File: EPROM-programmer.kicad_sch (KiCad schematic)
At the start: 63 parts, among them J1 ZIF-socket, J2 ISP, J3 DAC_VCC, J4 DAC_B, J5 GND, J6 Barrel_Jack_Switch, J7 VCC_SEL, J8 AMP_VCC, J9 GND, P1 USB-C, Q1 TIP41C, Q2 BC327, Q3 BC337, SW1 SW_Push, U1 ATmega1284-P, U2 MCP2221AxP, U3 MCP4812, U4 LM358, Y1 20M

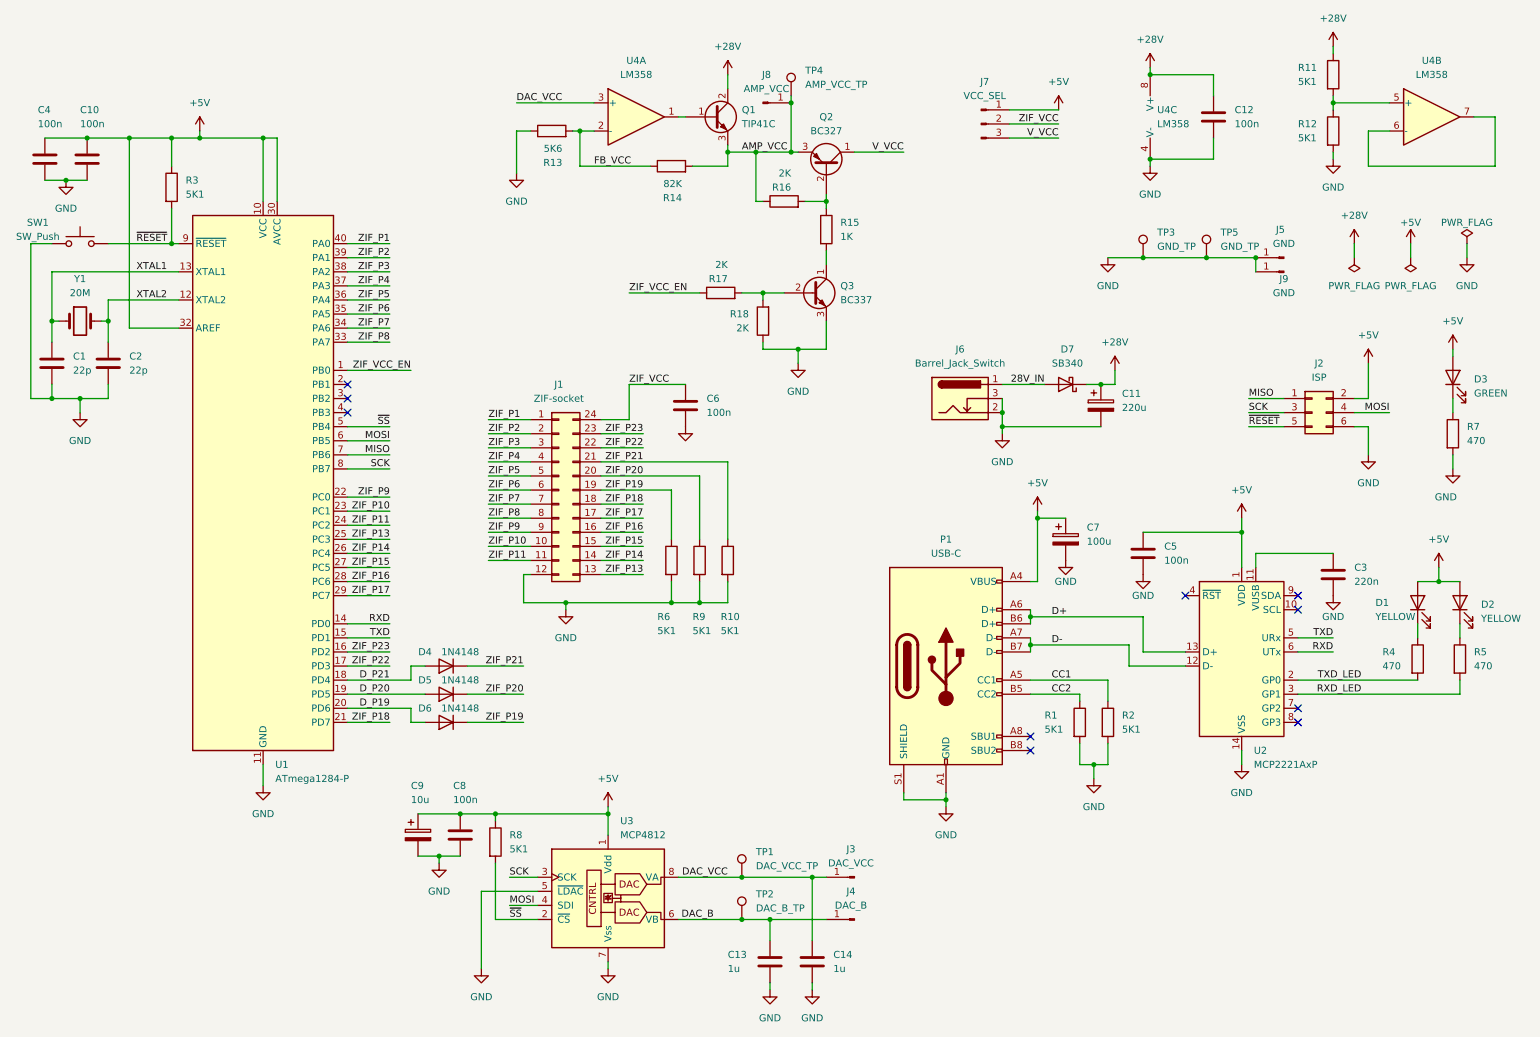
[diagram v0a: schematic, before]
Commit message: WIP use LM317
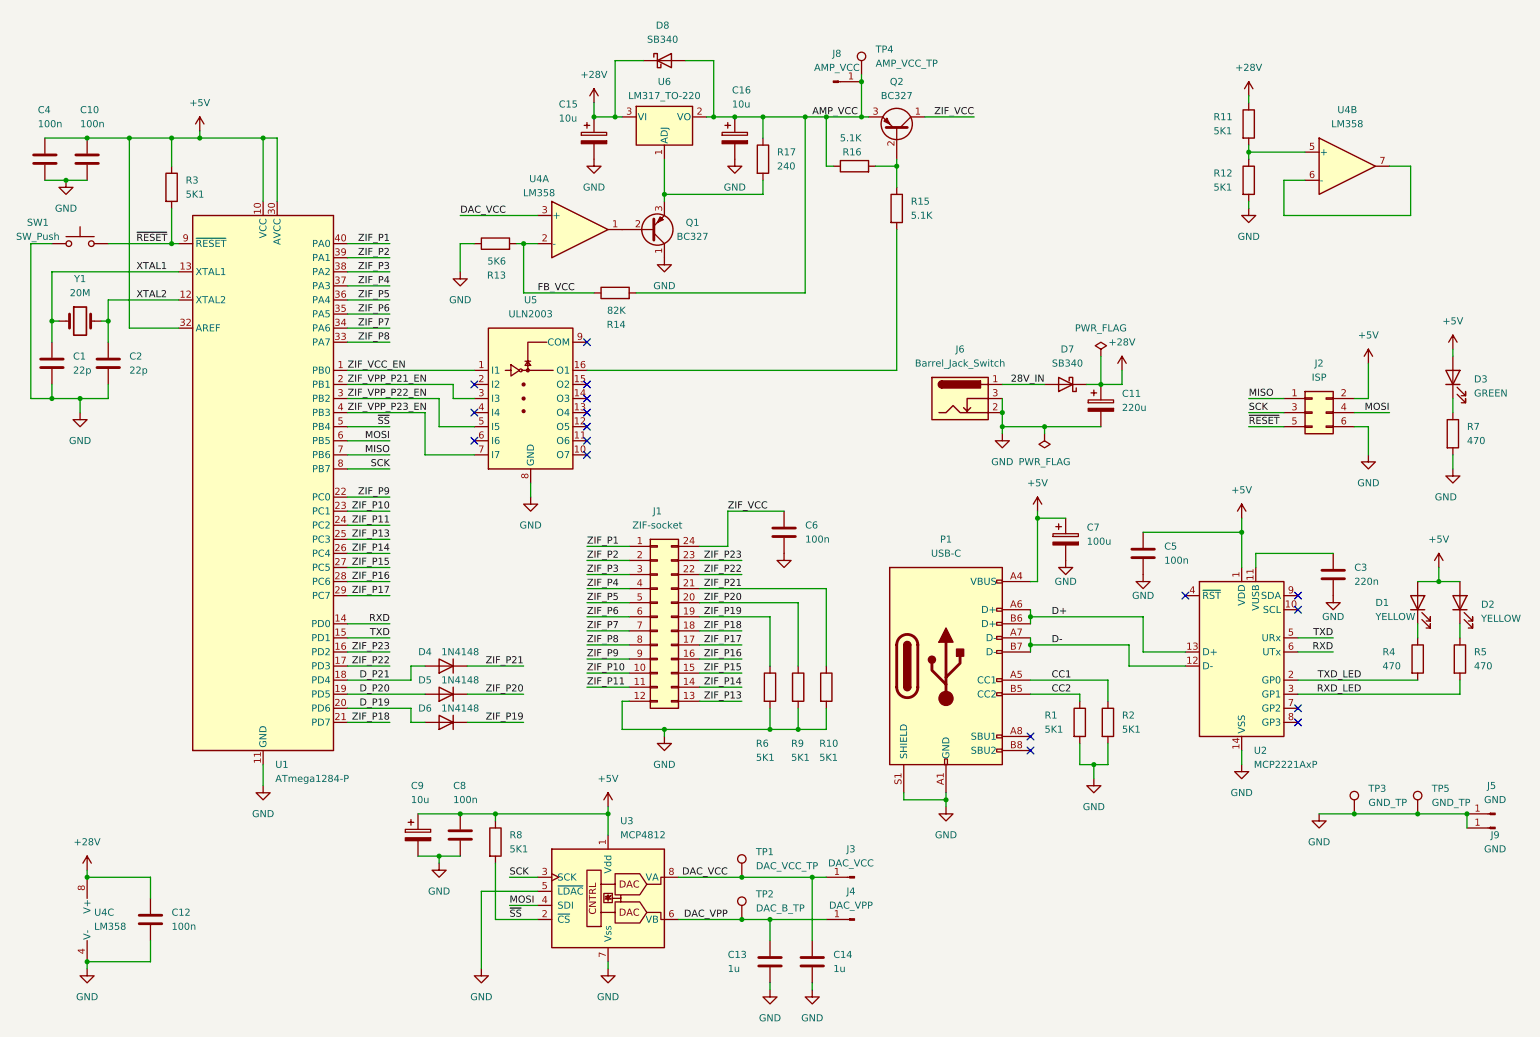
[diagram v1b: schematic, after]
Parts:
- removed J7: VCC_SEL, Connector_PinHeader_2.54mm:PinHeader_1x03_P2.54mm_Vertical, symbol Connector:Conn_01x03_Pin
- removed Q1: TIP41C, Package_TO_SOT_THT:TO-220-3_Vertical, symbol Transistor_BJT:TIP41C
- removed Q3: BC337, Package_TO_SOT_THT:TO-92_Inline_Wide, symbol Transistor_BJT:BC337
- removed R18: 2K, Resistor_THT:R_Axial_DIN0207_L6.3mm_D2.5mm_P10.16mm_Horizontal, symbol Device:R
- added C15, C16: 10u, Local:C_Rect_L4.6mm_W3.0mm_P2.50mm_MKS02_FKP02, symbol Device:C_Polarized
- added D8: SB340, Diode_THT:D_DO-201AD_P15.24mm_Horizontal, symbol Diode:B340
- added Q1: BC327, Package_TO_SOT_THT:TO-92_Inline_Wide, symbol Transistor_BJT:BC327
- added U5: ULN2003, Package_DIP:DIP-16_W7.62mm_Socket, symbol Transistor_Array:ULN2003
- added U6: LM317_TO-220, Package_TO_SOT_THT:TO-220-3_Vertical, symbol Regulator_Linear:LM317_TO-220
- J4: value DAC_B -> DAC_VPP
- R15: value 1K -> 5.1K
- R16: value 2K -> 5.1K
- R17: value 2K -> 240
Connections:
- net V_VCC is gone; now on net ZIF_VCC: Q2.1 (C)
- net +28V: now also C15.1, D8.1 (K), U6.3 (VI)
- net AMP_VCC: now also R17.1, C16.1, D8.2 (A), U6.2 (VO)
- net GND: now also C15.2, C16.2, Q1.1 (C), U5.8 (GND)
- net ZIF_VCC_EN: now also U5.1 (I1); no longer R17.1
- net ZIF_VPP_P21_EN: now reaches U1.2 (PB1)
- net ZIF_VPP_P21_EN: now also U5.3 (I3)
- net ZIF_VPP_P22_EN: now reaches U1.3 (PB2)
- net ZIF_VPP_P22_EN: now also U5.5 (I5)
- net ZIF_VPP_P23_EN: now reaches U1.4 (PB3)
- net ZIF_VPP_P23_EN: now also U5.7 (I7)
- net at R15.2: now also U5.16 (O1)
- net at R17.2: now also Q1.3 (E), U6.1 (ADJ)
- net at U4.1: now also Q1.2 (B)
- net DAC_B renamed DAC_VPP
- no-connect marks 10 -> 17
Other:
- moved on the sheet: C12, C6, J1, J5, J8, J9, Q2, R10, R11, R12, R13, R14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
